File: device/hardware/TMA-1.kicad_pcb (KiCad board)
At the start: 2 copper layers, 141.7 x 127.5 mm, 72 parts, among them J1 MAIN I/O, J2 I2C, Q1 2N3904, Q2 2N3904, Q3 2N3904, Q4 2N3904, Q5 2N3904, Q6 2N3904, Q7 2N3904, Q8 2N3904, SW1 CAN_{SW}, U1 STM32F407VETx, U2 NODEMCU32S, U3 MP1584EN-3.3, U4 LM393, U5 LM393, U6 ADXL345, U7 NEO-7M, U8 SN65HVD230

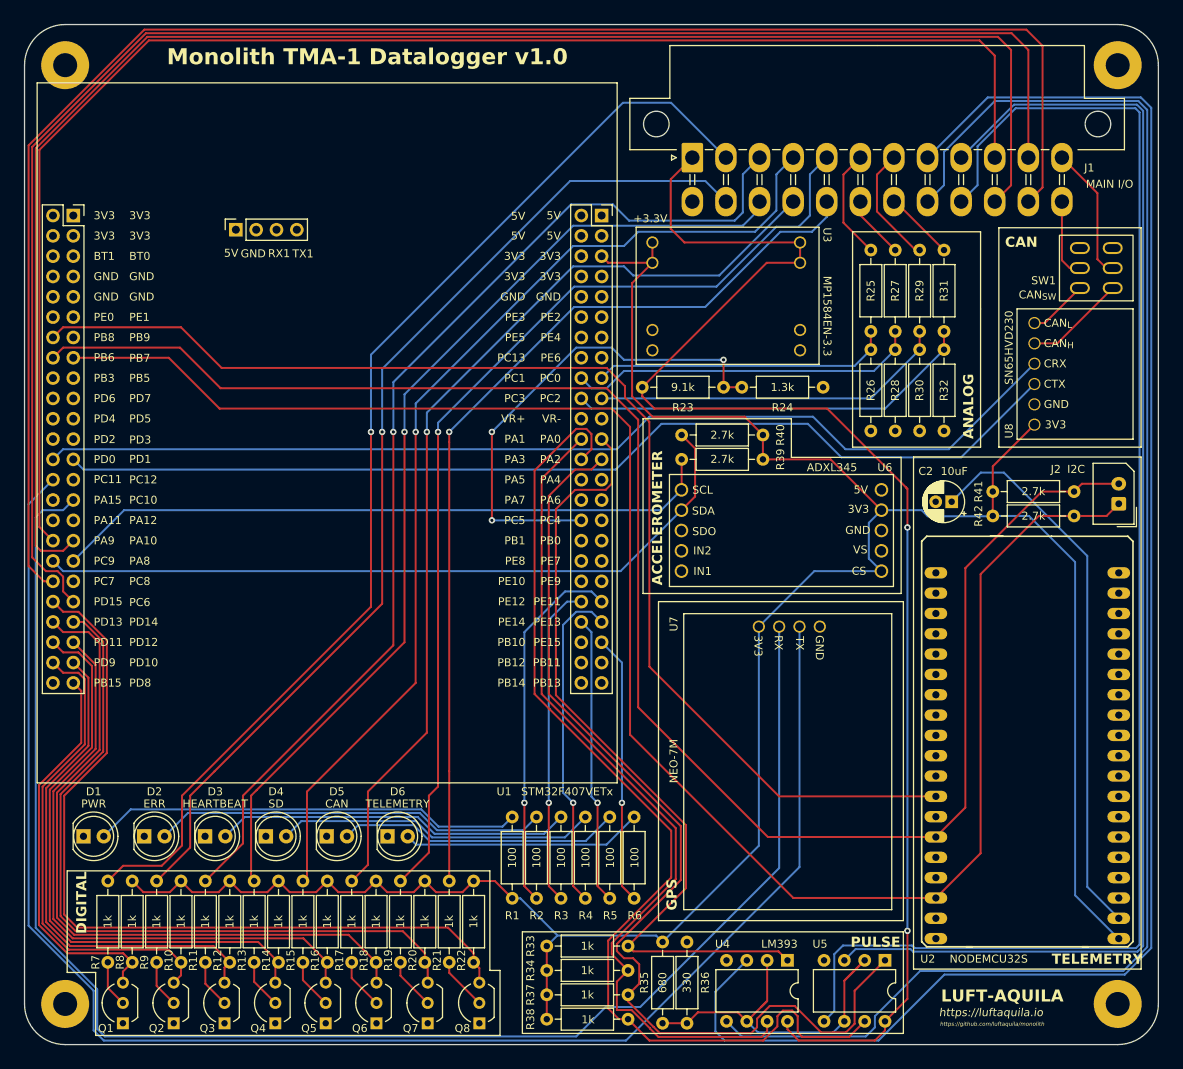
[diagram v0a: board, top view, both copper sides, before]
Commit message: add: PCB v1.0 gerber files
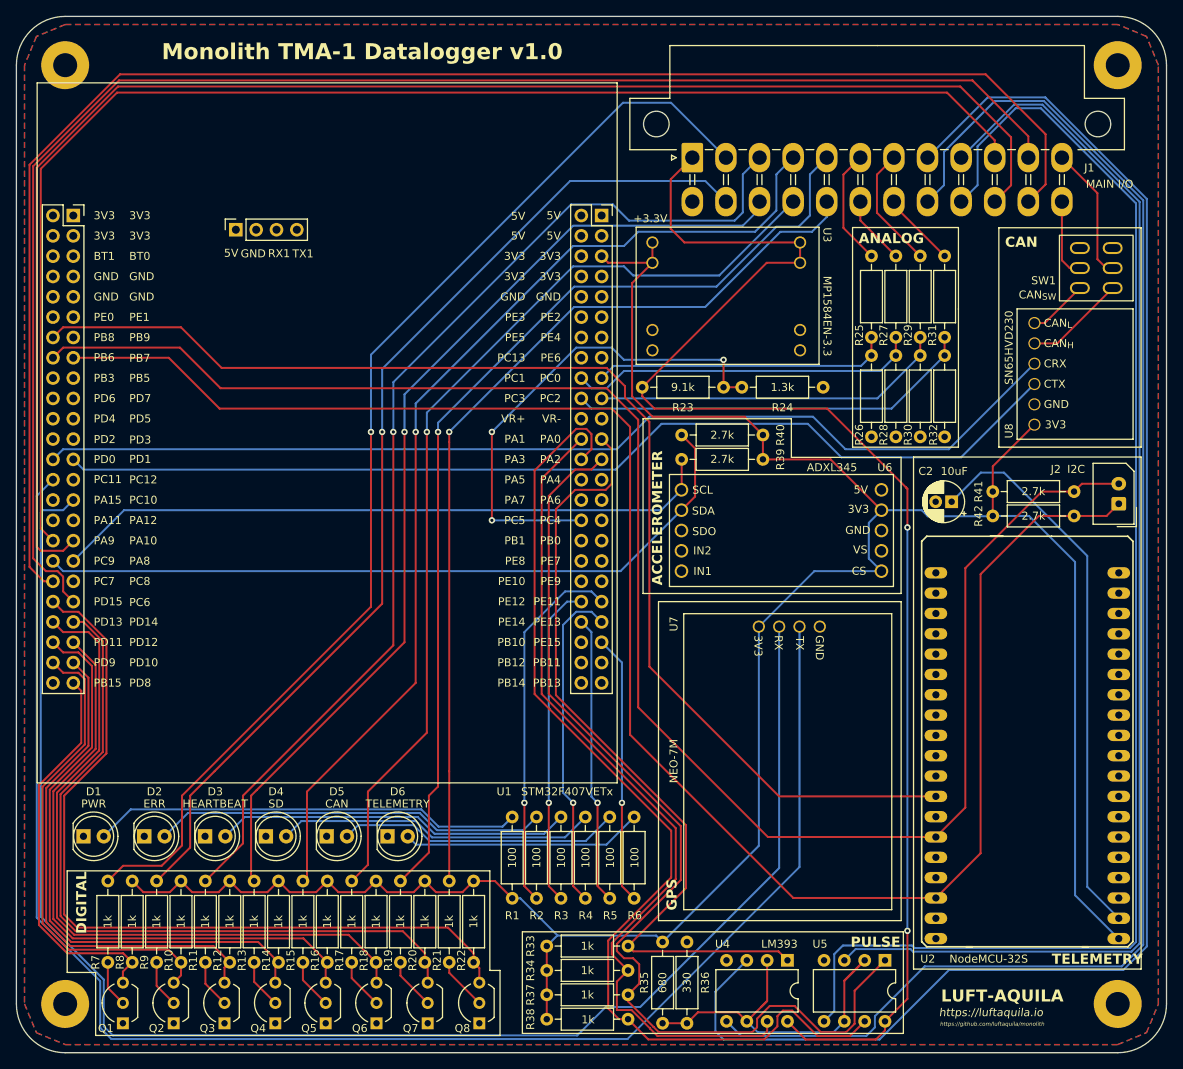
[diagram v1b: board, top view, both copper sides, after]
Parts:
- U2: value NODEMCU32S -> NodeMCU-32S
- moved R25 0.74 mm to (179.5, 59.5)
- moved R26 0.74 mm to (179.5, 72.0)
- moved R27 0.74 mm to (182.6, 59.5)
- moved R28 0.74 mm to (182.6, 72.0)
- moved R29 0.74 mm to (185.6, 59.5)
- moved R30 0.74 mm to (185.6, 72.0)
- moved R31 0.74 mm to (188.7, 59.5)
- moved R32 0.74 mm to (188.7, 72.0)
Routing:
- net /DEBUG_UART_TX: track 188.2 -> 174.9 mm
- net /DEBUG_UART_RX: track 203.3 -> 190.2 mm
- net /LOG_UART_TX: track 204.6 -> 191.8 mm
- net /LOG_UART_RX: track 210.2 -> 198.1 mm
- net /PIN0: track 206.9 -> 198.9 mm
- net /PIN1: track 199.0 -> 191.2 mm
- net /PIN3: track 182.1 -> 174.3 mm
- net /PIN2: track 168.6 -> 160.8 mm
- net /GPS_UART_RX: track 201.3 -> 199.6 mm
- net /STM_PIN3: track 130.2 -> 128.8 mm
- net /GPS_UART_TX: track 197.3 -> 196.0 mm
- net /AIN3: track 8.77 -> 9.62 mm
- net /AIN0: track 13.9 -> 14.6 mm
- net /AIN1: track 7.86 -> 8.63 mm
- net VBUS: track 177.9 -> 177.2 mm
- added copper zone on B.Cu, net GND
- added copper zone on F.Cu, net GND
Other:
- board size 141.7 x 127.5 mm -> 143.8 x 129.5 mm
